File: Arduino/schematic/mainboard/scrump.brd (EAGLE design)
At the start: 100 x 80 mm, 29 parts, among them J1 PINHEAD-FTSH, J2 USB-CON-5PIN-105017-0001, U1 ATSAMD21G-A, U2 LM3671, U3 MCP73831, Y1 32.768kHz

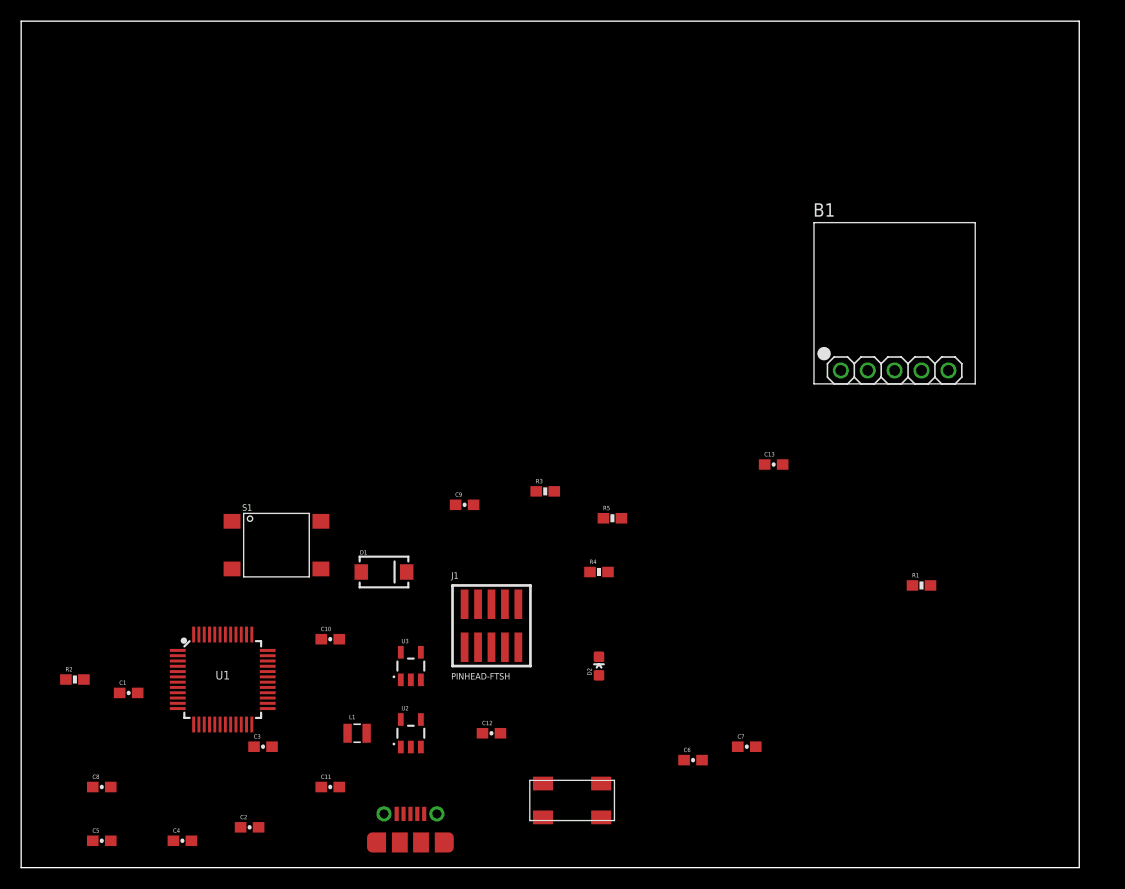
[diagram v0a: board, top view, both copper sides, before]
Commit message: Initial PCB
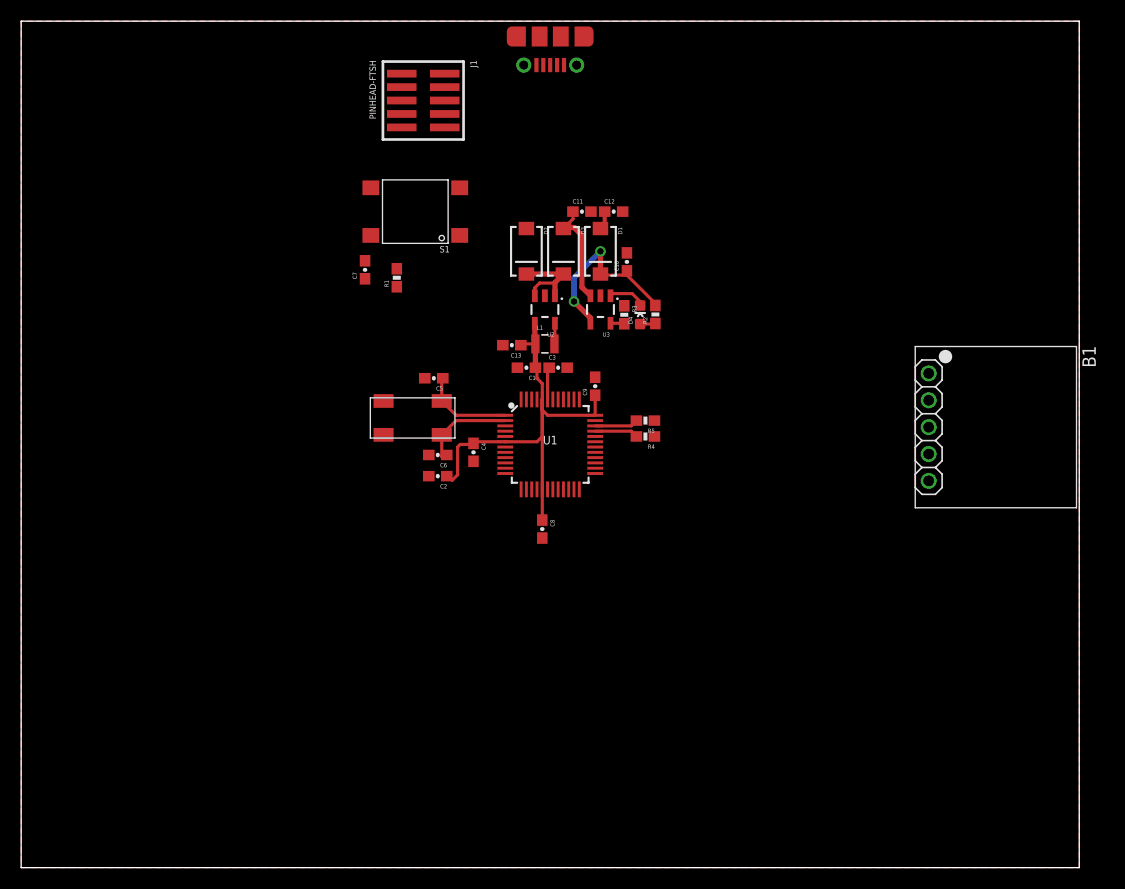
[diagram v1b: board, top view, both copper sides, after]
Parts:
- added D3: MBRA140, SparkFun-DiscreteSemi:SMA-DIODE
- added D4: RED 1.8V, SparkFun-LED:LED-0603
- C12: value 10uF -> 4.7uF
- C13: value 0.1uF -> 10uF
- C5: value 0.1uF -> 22pF
- C7: value 22pF -> 0.1uF
- C9: value 4.7uF -> 0.1uF
- D2: value RED 1.8V -> MBRA140; device SparkFun-LED:LED-0603 -> SparkFun-DiscreteSemi:SMA-DIODE
- L1: value 2.2uF -> 2.2uH
- R1: value 22R -> 330R
- R2: value 330R -> 1.5k
- R3: value 1.5k -> 5k
- R4: value 2k -> 22R
- moved J2 73.1 mm to (52.5, 75.8), turned to 180 degrees
- moved R2 64.8 mm to (59.9, 52.3), turned to 90 degrees
- moved C11 59.4 mm to (53.0, 62.0)
- moved C7 57.7 mm to (32.5, 56.5), turned to 90 degrees
- moved R1 57.5 mm to (35.5, 55.8), turned to 90 degrees
- moved C5 53.8 mm to (39.0, 46.2), turned to 180 degrees
- moved C12 50.6 mm to (56.0, 62.0)
- moved J1 50.1 mm to (38.0, 72.5), turned to 270 degrees
- moved C1 48.6 mm to (47.8, 47.2), turned to 180 degrees
- moved C8 48.2 mm to (49.2, 32.0), turned to 270 degrees
- moved C4 45.9 mm to (42.8, 39.2), turned to 270 degrees
- moved C3 45.4 mm to (50.8, 47.2)
- moved C10 45.4 mm to (57.2, 57.2), turned to 90 degrees
- moved U2 42.0 mm to (49.5, 52.8), turned to 180 degrees
- moved L1 40.9 mm to (49.5, 49.5)
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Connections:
- net PA02 renamed A0
- net PA03 renamed AREF
- net PA04 renamed A3
- net PA05 renamed A4
- net PA06 renamed D8
- net PA07 renamed D9
- net PA08 renamed D4
- net PA09 renamed D3
- net PA10 renamed D1
- net PA11 renamed D0
- net PA12 renamed MISO
- net PA14 renamed D2
- net PA15 renamed D5
- net PA16 renamed D11
- net PA17 renamed D13
- net PA18 renamed D10
- net PA19 renamed D12
- net PA20 renamed D6
- net PA21 renamed D7
- net PB02 renamed A5
- net PB08 renamed A1
- net PB09 renamed A2
- net PB10 renamed MOSI
- net PB11 renamed SCK
- net PB22 renamed TXD
- net PB23 renamed RXD
- removed net +5V: C11.1, D1.A, J2.1
- removed net PA00: C6.1, U1.1, Y1.P$1
- removed net PA01: C7.1, U1.2, Y1.P$4
- removed net VCC: C10.1, U2.1, U2.3, U3.3
- new net N$10: D2.C, D3.C, U2.1, U2.3
- new net V_BATT: C11.1, D3.A, U3.3
- new net V_USB: C12.1, D1.A, D2.A, J2.1
- new net XIN32: C5.1, U1.1, Y1.P$1
- new net XOUT32: C6.1, U1.2, Y1.P$4
- net +3V3: now also C8.1, C9.1; no longer C12.1, C5.1
- net D-: now also R4.2; no longer R1.2
- net GND: now also R3.1; no longer R4.1
- net N$2: now also R1.2; no longer R2.2
- net N$3: now also C10.1, R2.2; no longer C9.1, R3.2
- net N$6: now also D4.C; no longer D2.C
- net N$7: now also D4.A, R2.1; no longer D2.A, R3.1
- net N$8: now also R3.2; no longer R4.2
- net N$9: now also R4.1; no longer R1.1
- net RESET: now also C7.1, R1.1; no longer C8.1, R2.1
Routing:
- net +3V3: track 0.00 -> 44.3 mm
- net N$3: track 0.00 -> 17.6 mm, vias 0 -> 2
- net V_BATT: track 0.00 -> 10.1 mm
- net N$10: track 0.00 -> 9.92 mm
- net XOUT32: track 0.00 -> 9.11 mm
- net XIN32: track 0.00 -> 8.75 mm
- net D-: track 0.00 -> 4.11 mm
- net D+: track 0.00 -> 4.11 mm
- net N$6: track 0.00 -> 3.57 mm
- net N$1: track 0.00 -> 3.06 mm
- net N$5: track 0.00 -> 1.97 mm
- net V_USB: track 0.00 -> 1.77 mm
- net N$7: track 0.00 -> 1.46 mm
- net N$8: track 0.00 -> 1.32 mm
- added copper zone on layer 1, net GND
